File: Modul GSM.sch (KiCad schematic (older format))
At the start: 38 parts, among them K1 VBATT, K2 SMA, P1 STEROWNIK, Q1 BC847B, Q2 BC847B, Q3 BC847B, U1 74LS125, U2 LD1117S50TR, U3 SIM900D, U4 SIM

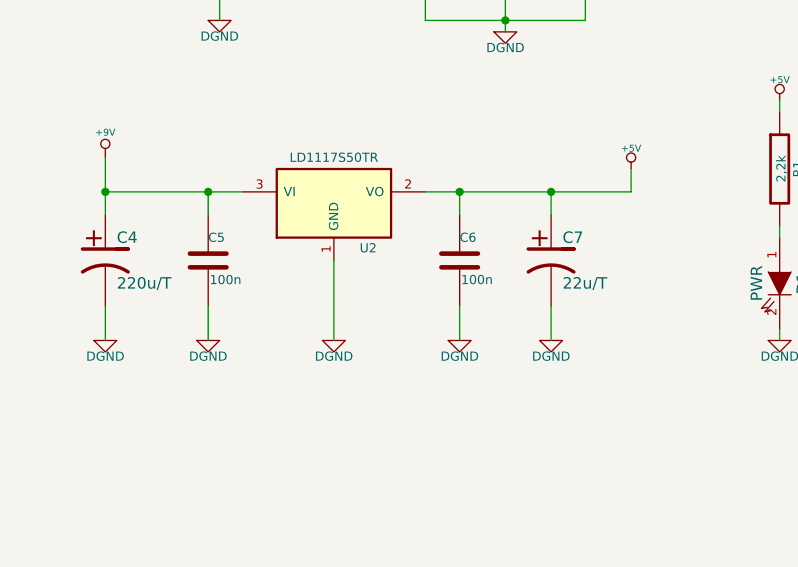
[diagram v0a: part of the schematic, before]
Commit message: Revert "Revert "28-03-2015""
This reverts commit a35226c248e7f072a54264f71b0718be7540caac.
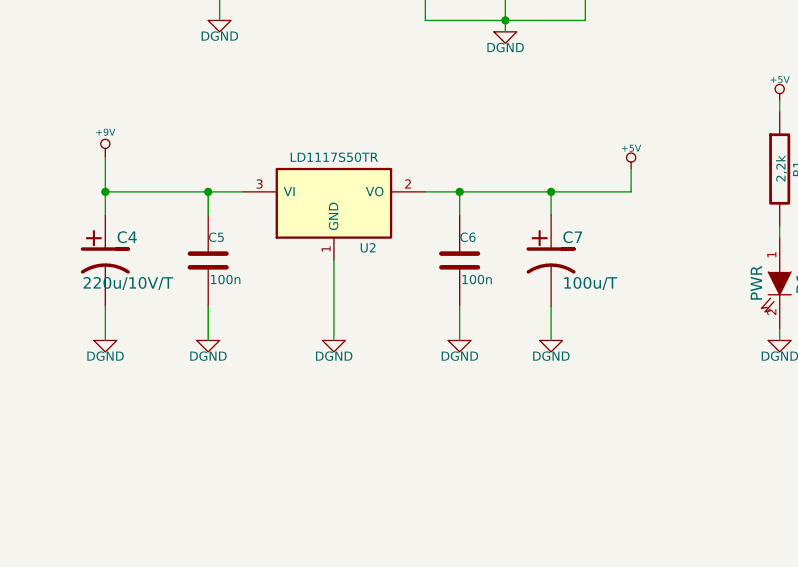
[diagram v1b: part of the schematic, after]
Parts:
- C4: value 220u/T -> 220u/10V/T
- C7: value 22u/T -> 100u/T
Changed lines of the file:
@@
 P 3450 2800
 F 0 "C7" H 3500 2900 50  0000 L CNN
-F 1 "22u/T" H 3500 2700 50  0000 L CNN
+F 1 "100u/T" H 3500 2700 50  0000 L CNN
 F 2 "~" H 3450 2800 60  0000 C CNN
 F 3 "~" H 3450 2800 60  0000 C CNN
@@
 P 1500 2800
 F 0 "C4" H 1550 2900 50  0000 L CNN
-F 1 "220u/T" H 1550 2700 50  0000 L CNN
+F 1 "220u/10V/T" H 1400 2700 50  0000 L CNN
 F 2 "~" H 1500 2800 60  0000 C CNN
 F 3 "~" H 1500 2800 60  0000 C CNN

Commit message: Revert "28-03-2015"
This reverts commit 6328e8af113ad8d7fc7daed5852ae822de97dd85.
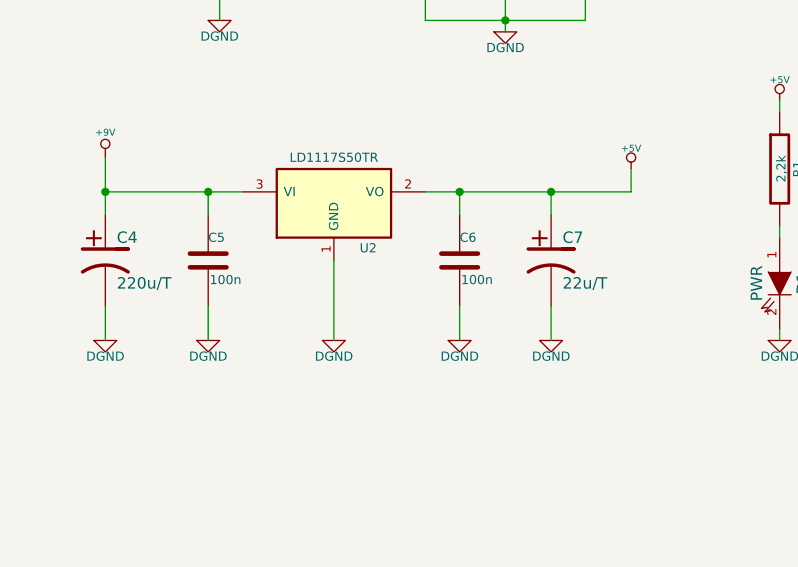
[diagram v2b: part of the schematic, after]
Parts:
- C4: value 220u/10V/T -> 220u/T
- C7: value 100u/T -> 22u/T
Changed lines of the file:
@@
 P 3450 2800
 F 0 "C7" H 3500 2900 50  0000 L CNN
-F 1 "100u/T" H 3500 2700 50  0000 L CNN
+F 1 "22u/T" H 3500 2700 50  0000 L CNN
 F 2 "~" H 3450 2800 60  0000 C CNN
 F 3 "~" H 3450 2800 60  0000 C CNN
@@
 P 1500 2800
 F 0 "C4" H 1550 2900 50  0000 L CNN
-F 1 "220u/10V/T" H 1400 2700 50  0000 L CNN
+F 1 "220u/T" H 1550 2700 50  0000 L CNN
 F 2 "~" H 1500 2800 60  0000 C CNN
 F 3 "~" H 1500 2800 60  0000 C CNN
